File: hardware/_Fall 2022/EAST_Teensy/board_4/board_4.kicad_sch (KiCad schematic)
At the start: 7 parts, among them J1 Conn_01x04, J2 Conn_02x09_Odd_Even, U1 Teensy4.1

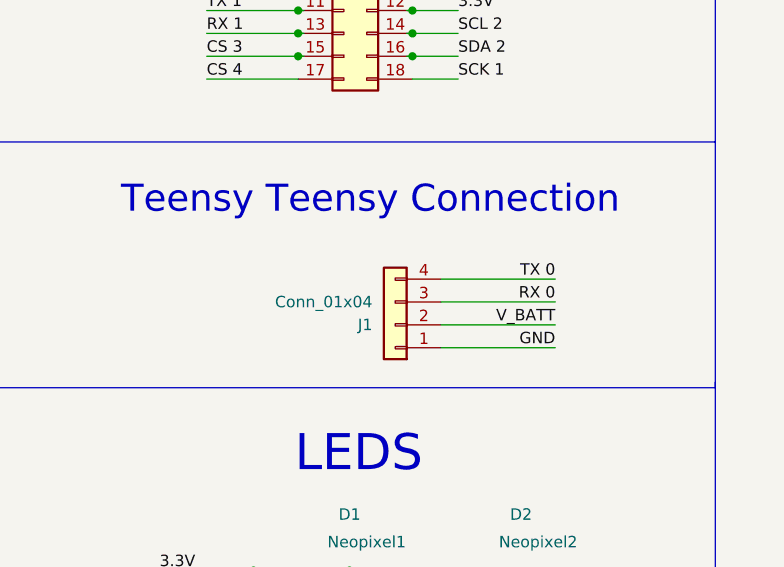
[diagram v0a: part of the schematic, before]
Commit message: minor fixes
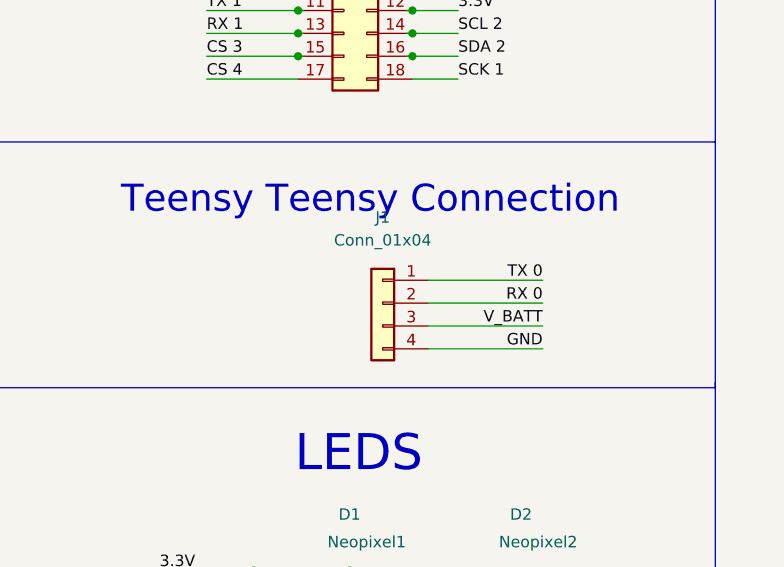
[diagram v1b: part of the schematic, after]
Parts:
- C1: JLC C307380 -> (none); Vendor (none) -> C14663
- C2: footprint Capacitor_SMD:C_0201_0603Metric -> Capacitor_SMD:C_0603_1608Metric; JLC C307380 -> (none); Vendor (none) -> C14663
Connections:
- net GND: now also J1.4 (Pin_4); no longer J1.1 (Pin_1)
- net RX 0: now also J1.2 (Pin_2); no longer J1.3 (Pin_3)
- net TX 0: now also J1.1 (Pin_1); no longer J1.4 (Pin_4)
- net V_BATT: now also J1.3 (Pin_3); no longer J1.2 (Pin_2)
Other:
- moved on the sheet: J1
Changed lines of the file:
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@@
     (stroke (width 0) (type default) (color 0 0 0 0))
   )
-  (wire (pts (xy 183.515 83.185) (xy 170.815 83.185))
+  (wire (pts (xy 182.118 83.312) (xy 169.418 83.312))
     (stroke (width 0) (type default) (color 0 0 0 0))
   )
@@
     (stroke (width 0) (type default) (color 0 0 0 0))
   )
-  (wire (pts (xy 183.515 80.645) (xy 170.815 80.645))
+  (wire (pts (xy 182.118 80.772) (xy 169.418 80.772))
     (stroke (width 0) (type default) (color 0 0 0 0))
   )
@@
     (stroke (width 0) (type default) (color 0 0 0 0))
   )
-  (wire (pts (xy 183.515 75.565) (xy 170.815 75.565))
+  (wire (pts (xy 182.118 75.692) (xy 169.418 75.692))
     (stroke (width 0) (type default) (color 0 0 0 0))
   )
@@
     (stroke (width 0) (type default) (color 0 0 0 0))
   )
-  (wire (pts (xy 183.515 78.105) (xy 170.815 78.105))
+  (wire (pts (xy 182.118 78.232) (xy 169.418 78.232))
     (stroke (width 0) (type default) (color 0 0 0 0))
   )
@@
     (effects (font (size 1.27 1.27)) (justify right bottom))
   )
-  (label "RX 0" (at 183.515 78.105 180)
+  (label "RX 0" (at 182.118 78.232 180)
     (effects (font (size 1.27 1.27)) (justify right bottom))
   )
@@
     (effects (font (size 1.27 1.27)) (justify left bottom))
   )
-  (label "V_BATT" (at 183.515 80.645 180)
+  (label "V_BATT" (at 182.118 80.772 180)
     (effects (font (size 1.27 1.27)) (justify right bottom))
   )
@@
     (effects (font (size 1.27 1.27)) (justify left bottom))
   )
-  (label "GND" (at 183.515 83.185 180)
+  (label "GND" (at 182.118 83.312 180)
     (effects (font (size 1.27 1.27)) (justify right bottom))
   )
@@
     (effects (font (size 1.27 1.27)) (justify left bottom))
   )
-  (label "TX 0" (at 183.515 75.565 180)
+  (label "TX 0" (at 182.118 75.692 180)
     (effects (font (size 1.27 1.27)) (justify right bottom))
   )
@@
       (effects (font (size 1.27 1.27)) (justify left))
     )
-    (property "Footprint" "Capacitor_SMD:C_0201_0603Metric" (id 2) (at 149.0218 114.427 0)
+    (property "Footprint" "Capacitor_SMD:C_0603_1608Metric" (id 2) (at 149.0218 114.427 0)
       (effects (font (size 1.27 1.27)) hide)
     )
@@
       (effects (font (size 1.27 1.27)) hide)
     )
-    (property "JLC" "C307380" (id 4) (at 149.987 118.237 0)
+    (property "Vendor" "C14663" (id 4) (at 149.987 118.237 0)
       (effects (font (size 1.27 1.27)) hide)
     )
@@
       (effects (font (size 1.27 1.27)) hide)
     )
-    (property "JLC" "C307380" (id 4) (at 109.22 69.85 0)
+    (property "Vendor" "C14663" (id 4) (at 109.22 69.85 0)
       (effects (font (size 1.27 1.27)) hide)
     )
@@
     (pin "1")
   )
-  (symbol (lib_id "Connector_Generic:Conn_01x04") (at 165.735 80.645 180) (unit 1)
+  (symbol (lib_id "Connector_Generic:Conn_01x04") (at 164.338 78.232 0) (mirror y) (unit 1)
     (in_bom yes) (on_board yes) (fields_autoplaced)
-    (property "Reference" "J1" (id 0) (at 163.195 80.6451 0)
-      (effects (font (size 1.27 1.27)) (justify left))
-    )
-    (property "Value" "Conn_01x04" (id 1) (at 163.195 78.1051 0)
-      (effects (font (size 1.27 1.27)) (justify left))
-    )
-    (property "Footprint" "Connector_JST:JST_PH_S4B-PH-K_1x04_P2.00mm_Horizontal" (id 2) (at 165.735 80.645 0)
-      (effects (font (size 1.27 1.27)) hide)
-    )
-    (property "Datasheet" "~" (id 3) (at 165.735 80.645 0)
+    (property "Reference" "J1" (id 0) (at 164.338 68.707 0))
+    (property "Value" "Conn_01x04" (id 1) (at 164.338 71.247 0))
+    (property "Footprint" "Connector_JST:JST_PH_S4B-PH-K_1x04_P2.00mm_Horizontal" (id 2) (at 164.338 78.232 0)
+      (effects (font (size 1.27 1.27)) hide)
+    )
+    (property "Datasheet" "~" (id 3) (at 164.338 78.232 0)
       (effects (font (size 1.27 1.27)) hide)
     )
@@
     )
     (path "/509c503b-65f7-47ea-a38c-398e1359983b"
-      (reference "C2") (unit 1) (value "0.1uf") (footprint "Capacitor_SMD:C_0201_0603Metric")
+      (reference "C2") (unit 1) (value "0.1uf") (footprint "Capacitor_SMD:C_0603_1608Metric")
     )
     (path "/b88239bc-ae48-46ce-a575-bdfc495bad18"
